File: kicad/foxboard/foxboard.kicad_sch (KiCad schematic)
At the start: 183 parts, among them J2 USB_C_Receptacle_USB2.0, K1 KEYSW, K10 KEYSW, K11 KEYSW, K12 KEYSW, K13 KEYSW, K14 KEYSW, K15 KEYSW, K16 KEYSW, K17 KEYSW, K18 KEYSW, K19 KEYSW, K2 KEYSW, K20 KEYSW, K21 KEYSW, K22 KEYSW, K23 KEYSW, K24 KEYSW, K25 KEYSW, K26 KEYSW, K27 KEYSW, K28 KEYSW, K29 KEYSW, K3 KEYSW, K30 KEYSW, K31 KEYSW, K32 KEYSW, K33 KEYSW, K34 KEYSW, K35 KEYSW, K36 KEYSW, K37 KEYSW, K38 KEYSW, K39 KEYSW, K4 KEYSW, K40 KEYSW, K41 KEYSW, K42 KEYSW, K43 KEYSW, K44 KEYSW, K45 KEYSW, K46 KEYSW, K47 KEYSW, K48 KEYSW, K49 KEYSW, K5 KEYSW, K50 KEYSW, K51 KEYSW, K52 KEYSW, K53 KEYSW, K54 KEYSW, K55 KEYSW, K56 KEYSW, K57 KEYSW, K58 KEYSW, K59 KEYSW, K6 KEYSW, K60 KEYSW, K61 KEYSW, K62 KEYSW, K63 KEYSW, K64 KEYSW, K65 KEYSW, K66 KEYSW, K67 KEYSW, K68 KEYSW, K69 KEYSW, K7 KEYSW, K70 KEYSW, K71 KEYSW, K72 KEYSW, K73 KEYSW, K74 KEYSW, K75 KEYSW, K76 KEYSW, K77 KEYSW, K78 KEYSW, K79 KEYSW, K8 KEYSW, K80 KEYSW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

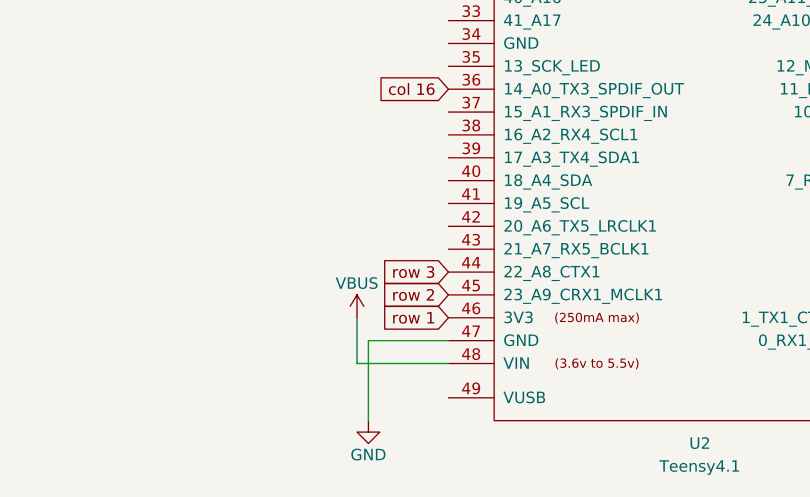
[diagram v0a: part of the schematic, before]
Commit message: update
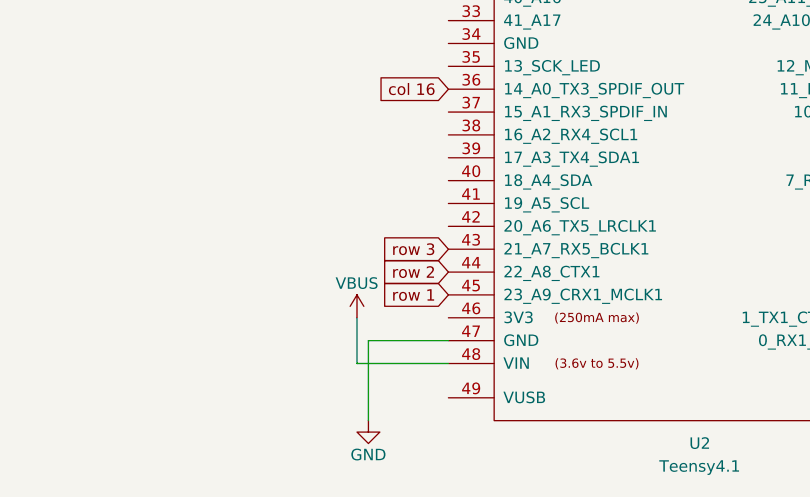
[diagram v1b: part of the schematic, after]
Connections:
- net row 1: now also U2.45 (23_A9_CRX1_MCLK1); no longer U2.46 (3V3)
- net row 2: now also U2.44 (22_A8_CTX1); no longer U2.45 (23_A9_CRX1_MCLK1)
- net row 3: now also U2.43 (21_A7_RX5_BCLK1); no longer U2.44 (22_A8_CTX1)
